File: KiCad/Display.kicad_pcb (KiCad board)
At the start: 2 copper layers, 44.5 x 67 mm, 30 parts, among them J1 DC, J2 USB-C, M1 OLED1.5-RGB, U1 L86-M33, U2 ESP32-PICO-MINI-02, U3 FT231XQ, U4 LMR16006+FB, U5 QR

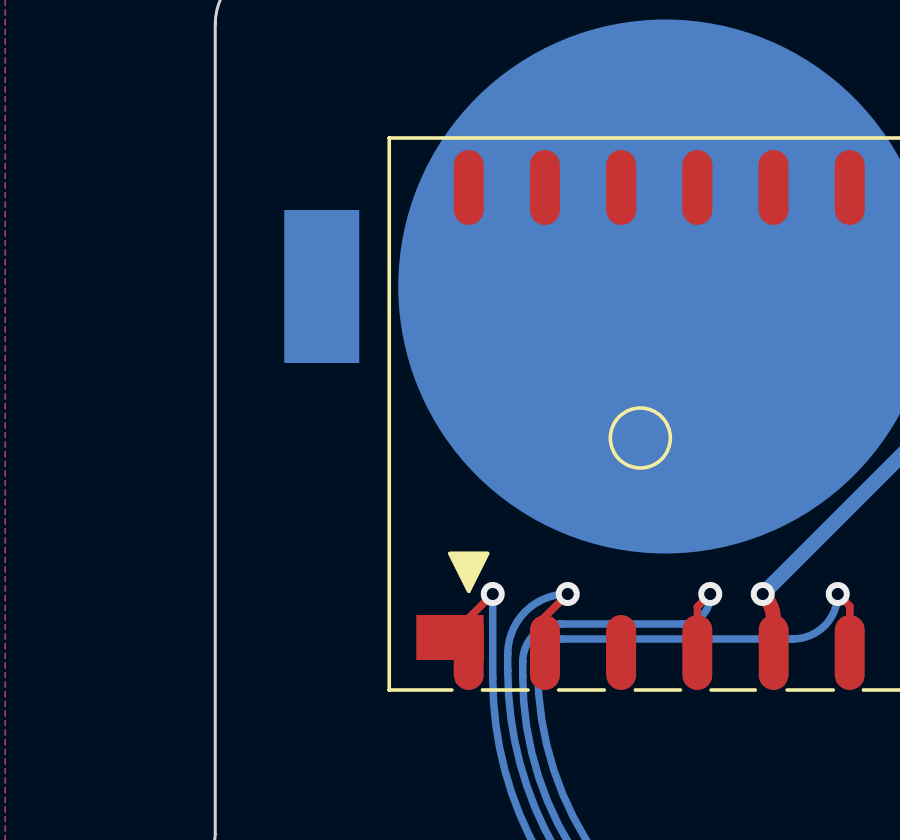
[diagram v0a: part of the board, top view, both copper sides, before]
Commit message: Resistors
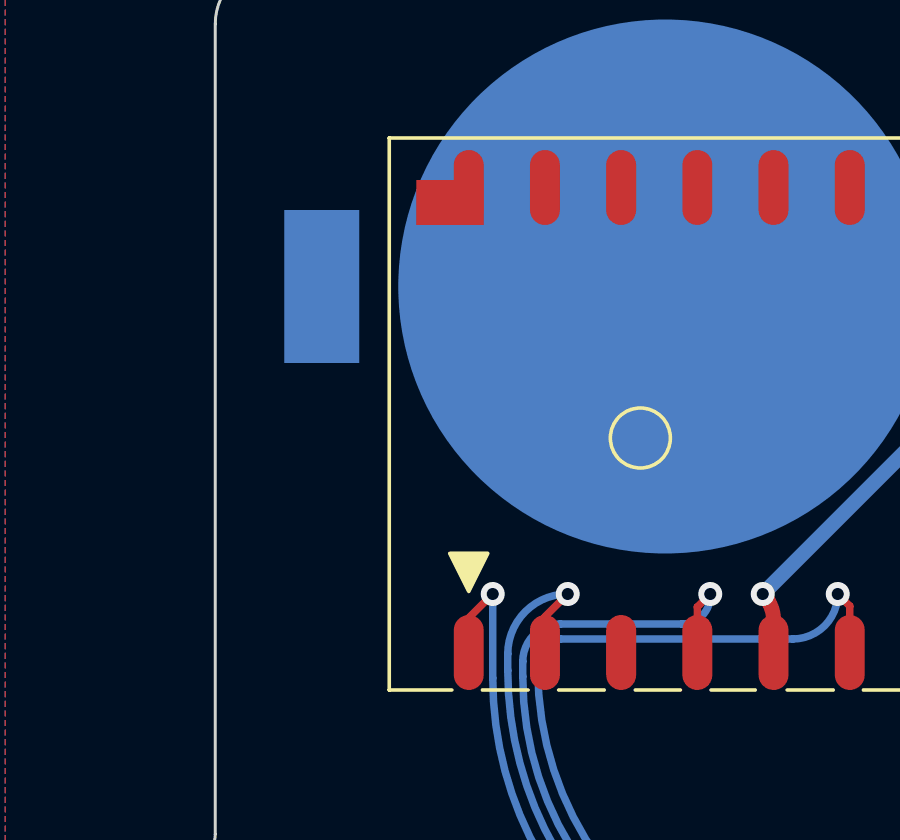
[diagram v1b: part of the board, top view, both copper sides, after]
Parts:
- R12: value 3M 1% or NF -> 30k 1% or NF
- R8: value 10M 1% or 0R -> 100k 1% or 0R
